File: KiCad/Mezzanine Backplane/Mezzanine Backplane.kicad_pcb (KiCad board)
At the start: 4 copper layers, 29.1 x 85 mm, 9 parts, among them J1 BB0500220F-1002C-001, J2 BB0500220F-1002C-001, J3 Conn_02x25_Odd_Even, J4 Conn_02x25_Odd_Even

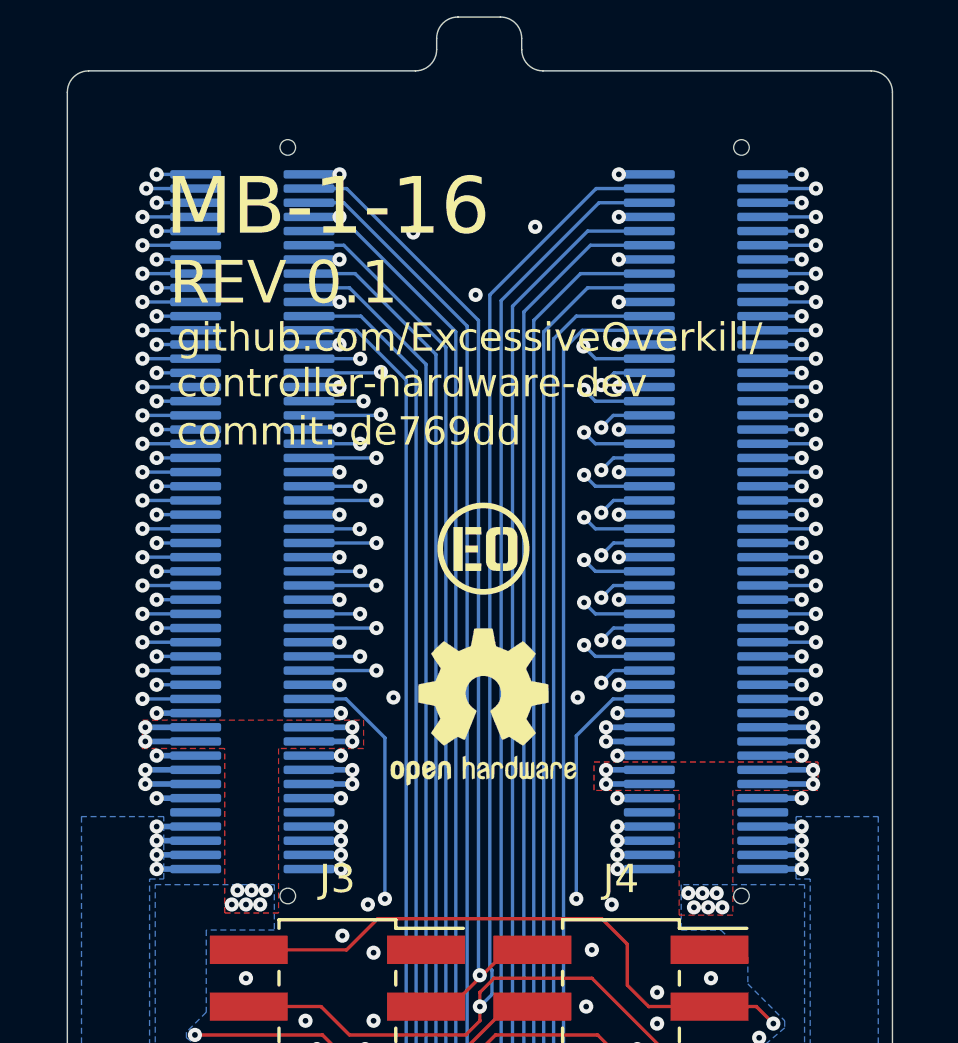
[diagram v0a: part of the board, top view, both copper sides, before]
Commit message: update
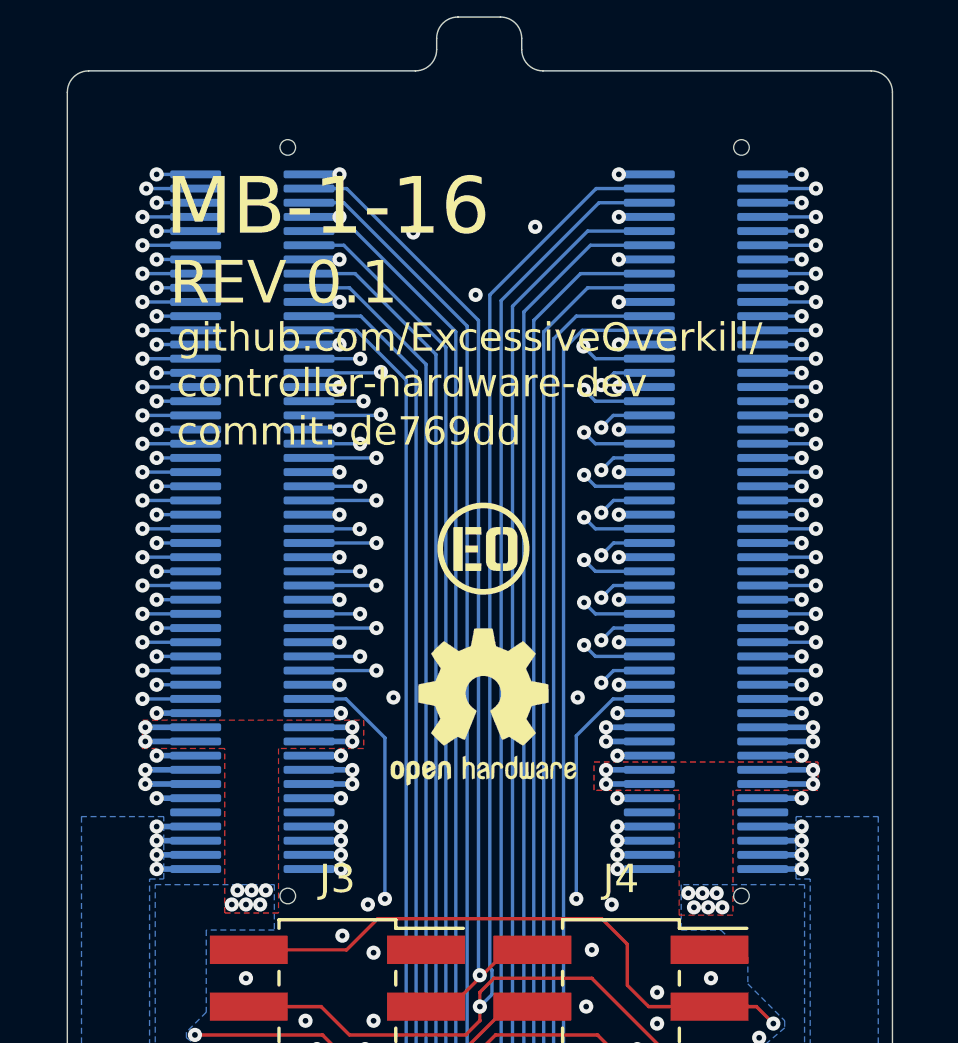
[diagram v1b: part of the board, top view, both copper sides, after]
